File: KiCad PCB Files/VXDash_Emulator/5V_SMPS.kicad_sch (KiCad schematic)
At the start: 13 parts, among them IC1 AP62200

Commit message: Emulator board : BOM and fab prep
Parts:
- C3: MFT (none) -> Samsung Electro-Mechanics; MFT_PN (none) -> CL31B106KAHNNNE
- C4, C5, C7: MFT (none) -> Samsung Electro-Mechanics; MFT_PN (none) -> CL10B104KB8NNWC
- C6: MFT (none) -> Kyocera AVX; MFT_PN (none) -> 06035C220JAT2A
- C8, C9: MFT (none) -> Samsung Electro-Mechanics; MFT_PN (none) -> CL31B226KPHNNNE
- R42: MFT (none) -> Yageo; MFT_PN (none) -> RC0603FR-071KL
- R43: MFT (none) -> StackPole Electronics; MFT_PN (none) -> RMCF0603FT100K
- R44: MFT (none) -> Yageo; MFT_PN (none) -> RC0603FR-0743KL
- R45: MFT (none) -> Yageo; MFT_PN (none) -> RC0603FR-078K2L
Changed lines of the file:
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@@
 			)
 		)
-		(property "Description" ""
+		(property "Description" "CAP CER 22PF 50V X7R 0603"
 			(at 157.48 86.36 0)
 			(effects
@@
 			)
 		)
-		(property "MFT" ""
+		(property "MFT" "Kyocera AVX"
 			(at 157.48 86.36 0)
 			(effects
@@
 			)
 		)
-		(property "MFT_PN" ""
+		(property "MFT_PN" "06035C220JAT2A"
 			(at 157.48 86.36 0)
 			(effects
@@
 			)
 		)
-		(property "Description" ""
+		(property "Description" "CAP CER 0.1UF 50V X7R 0603"
 			(at 90.17 82.55 0)
 			(effects
@@
 			)
 		)
-		(property "MFT" ""
+		(property "MFT" "Samsung Electro-Mechanics"
 			(at 90.17 82.55 0)
 			(effects
@@
 			)
 		)
-		(property "MFT_PN" ""
+		(property "MFT_PN" "CL10B104KB8NNWC"
 			(at 90.17 82.55 0)
 			(effects
@@
 			)
 		)
-		(property "Description" ""
+		(property "Description" "CAP CER 22UF 10V X7R 1206"
 			(at 189.23 86.36 0)
 			(effects
@@
 			)
 		)
-		(property "MFT" ""
+		(property "MFT" "Samsung Electro-Mechanics"
 			(at 189.23 86.36 0)
 			(effects
@@
 			)
 		)
-		(property "MFT_PN" ""
+		(property "MFT_PN" "CL31B226KPHNNNE"
 			(at 189.23 86.36 0)
 			(effects
@@
 			)
 		)
-		(property "Description" ""
+		(property "Description" "CAP CER 22UF 10V X7R 1206"
 			(at 181.61 86.36 0)
 			(effects
@@
 			)
 		)
-		(property "MFT" ""
+		(property "MFT" "Samsung Electro-Mechanics"
 			(at 181.61 86.36 0)
 			(effects
@@
 			)
 		)
-		(property "MFT_PN" ""
+		(property "MFT_PN" "CL31B226KPHNNNE"
 			(at 181.61 86.36 0)
 			(effects
@@
 			)
 		)
-		(property "Description" ""
+		(property "Description" "RES 1K OHM 1% 1/10W 0603"
 			(at 74.93 91.44 0)
 			(effects
@@
 			)
 		)
-		(property "MFT" ""
+		(property "MFT" "Yageo"
 			(at 74.93 91.44 0)
 			(effects
@@
 			)
 		)
-		(property "MFT_PN" ""
+		(property "MFT_PN" "RC0603FR-071KL"
 			(at 74.93 91.44 0)
 			(effects
@@
 			)
 		)
-		(property "Description" ""
+		(property "Description" "FIXED IND 4.7UH 3.2A 32 MOHM SMD"
 			(at 142.24 83.82 0)
 			(effects
@@
 			)
 		)
-		(property "Description" ""
+		(property "Description" "CAP CER 0.1UF 50V X7R 0603"
 			(at 129.54 76.2 0)
 			(effects
@@
 			)
 		)
-		(property "MFT" ""
+		(property "MFT" "Samsung Electro-Mechanics"
 			(at 129.54 76.2 0)
 			(effects
@@
 			)
 		)
-		(property "MFT_PN" ""
+		(property "MFT_PN" "CL10B104KB8NNWC"
 			(at 129.54 76.2 0)
 			(effects
@@
 			)
 		)
-		(property "Description" ""
+		(property "Description" "CAP CER 0.1UF 50V X7R 0603"
 			(at 173.99 86.36 0)
 			(effects
@@
 			)
 		)
-		(property "MFT" ""
+		(property "MFT" "Samsung Electro-Mechanics"
 			(at 173.99 86.36 0)
 			(effects
@@
 			)
 		)
-		(property "MFT_PN" ""
+		(property "MFT_PN" "CL10B104KB8NNWC"
 			(at 173.99 86.36 0)
 			(effects
@@
 			)
 		)
-		(property "Description" ""
+		(property "Description" "RES 8.2K OHM 1% 1/10W 0603"
 			(at 148.59 97.79 0)
 			(effects
@@
 			)
 		)
-		(property "MFT" ""
+		(property "MFT" "Yageo"
 			(at 148.59 97.79 0)
 			(effects
@@
 			)
 		)
-		(property "MFT_PN" ""
+		(property "MFT_PN" "RC0603FR-078K2L"
 			(at 148.59 97.79 0)
 			(effects
@@
 			)
 		)
-		(property "Description" ""
+		(property "Description" "CAP CER 10UF 25V X7R 1206"
 			(at 82.55 82.55 0)
 			(effects
@@
 			)
 		)
-		(property "MFT" ""
+		(property "MFT" "Samsung Electro-Mechanics"
 			(at 82.55 82.55 0)
 			(effects
@@
 			)
 		)
-		(property "MFT_PN" ""
+		(property "MFT_PN" "CL31B106KAHNNNE"
 			(at 82.55 82.55 0)
 			(effects
@@
 			)
 		)
-		(property "Description" ""
+		(property "Description" "RES 100K OHM 1% 1/10W 0603"
 			(at 100.33 96.52 0)
 			(effects
@@
 			)
 		)
-		(property "MFT" ""
+		(property "MFT" "StackPole Electronics"
 			(at 100.33 96.52 0)
 			(effects
@@
 			)
 		)
-		(property "MFT_PN" ""
+		(property "MFT_PN" "RMCF0603FT100K"
 			(at 100.33 96.52 0)
 			(effects
@@
 			)
 		)
-		(property "Description" ""
+		(property "Description" "RES 43K OHM 1% 1/10W 0603"
 			(at 148.59 86.36 0)
 			(effects
@@
 			)
 		)
-		(property "MFT" ""
+		(property "MFT" "Yageo"
 			(at 148.59 86.36 0)
 			(effects
@@
 			)
 		)
-		(property "MFT_PN" ""
+		(property "MFT_PN" "RC0603FR-0743KL"
 			(at 148.59 86.36 0)
 			(effects

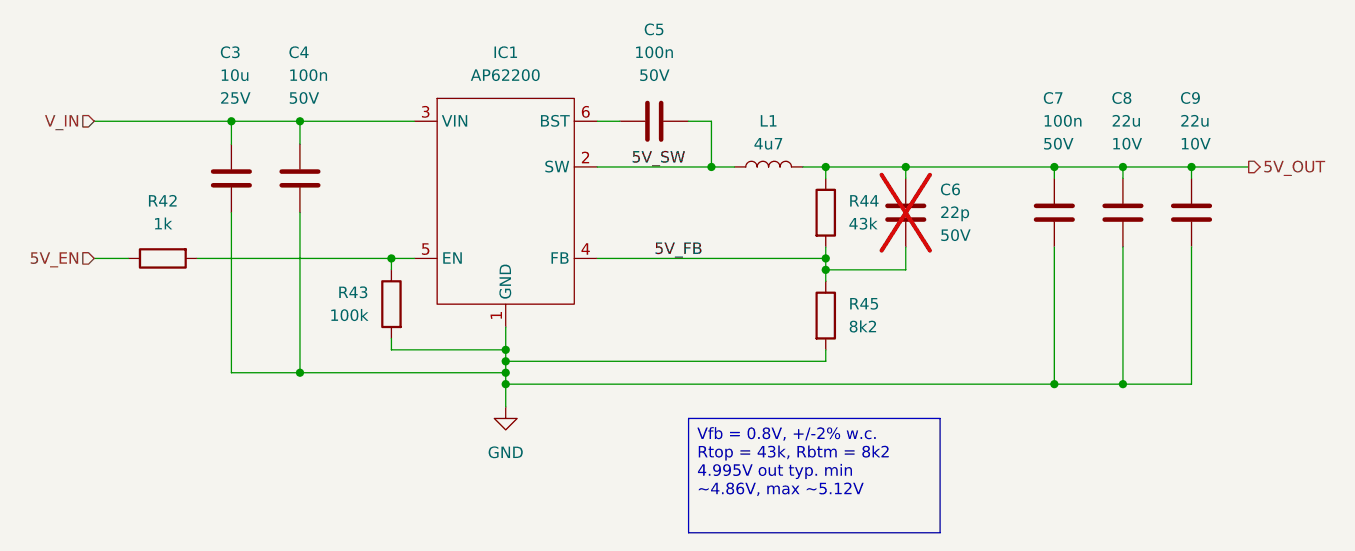
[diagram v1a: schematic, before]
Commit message: Emulator : LCSC part numbers and production files
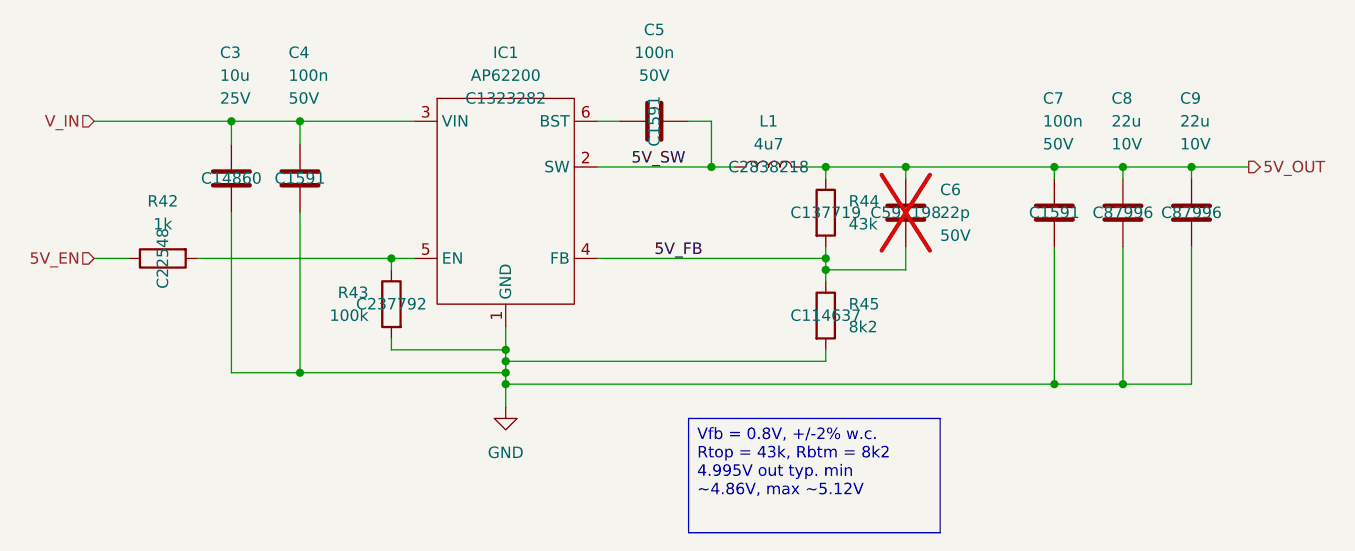
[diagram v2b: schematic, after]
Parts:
- C3: LCSC (none) -> C14860
- C4, C5, C7: LCSC (none) -> C1591; MFT_PN CL10B104KB8NNWC -> CL10B104KB8NNNC
- C6: LCSC (none) -> C597198
- C8, C9: LCSC (none) -> C87996
- IC1: LCSC (none) -> C1323282
- L1: LCSC (none) -> C2838218
- R42: LCSC (none) -> C22548
- R43: LCSC (none) -> C237792
- R44: LCSC (none) -> C137719
- R45: LCSC (none) -> C114637
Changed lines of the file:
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@@
+			)
+		)
+		(property "LCSC" "C597198"
+			(at 157.48 86.36 0)
+			(effects
+				(font
+					(size 1.27 1.27)
+				)
 			)
 		)
@@
 			)
 		)
-		(property "MFT_PN" "CL10B104KB8NNWC"
+		(property "MFT_PN" "CL10B104KB8NNNC"
 			(at 90.17 82.55 0)
 			(effects
@@
 				)
 				(hide yes)
+			)
+		)
+		(property "LCSC" "C1591"
+			(at 90.17 82.55 0)
+			(effects
+				(font
+					(size 1.27 1.27)
+				)
 			)
 		)
@@
 			)
 		)
+		(property "LCSC" "C87996"
+			(at 189.23 86.36 0)
+			(effects
+				(font
+					(size 1.27 1.27)
+				)
+			)
+		)
 		(pin "2"
 		)
@@
 				)
 				(hide yes)
+			)
+		)
+		(property "LCSC" "C87996"
+			(at 181.61 86.36 0)
+			(effects
+				(font
+					(size 1.27 1.27)
+				)
 			)
 		)
@@
 				)
 				(hide yes)
+			)
+		)
+		(property "LCSC" "C1323282"
+			(at 113.03 73.66 0)
+			(effects
+				(font
+					(size 1.27 1.27)
+				)
 			)
 		)
@@
 			)
 		)
+		(property "LCSC" "C22548"
+			(at 74.93 91.44 0)
+			(effects
+				(font
+					(size 1.27 1.27)
+				)
+			)
+		)
 		(pin "1"
 		)
@@
 				)
 				(hide yes)
+			)
+		)
+		(property "LCSC" "C2838218"
+			(at 142.24 81.28 0)
+			(effects
+				(font
+					(size 1.27 1.27)
+				)
 			)
 		)
@@
 			)
 		)
-		(property "MFT_PN" "CL10B104KB8NNWC"
+		(property "MFT_PN" "CL10B104KB8NNNC"
 			(at 129.54 76.2 0)
 			(effects
@@
 				)
 				(hide yes)
+			)
+		)
+		(property "LCSC" "C1591"
+			(at 129.54 76.2 0)
+			(effects
+				(font
+					(size 1.27 1.27)
+				)
 			)
 		)
@@
 			)
 		)
-		(property "MFT_PN" "CL10B104KB8NNWC"
+		(property "MFT_PN" "CL10B104KB8NNNC"
 			(at 173.99 86.36 0)
 			(effects
@@
 				)
 				(hide yes)
+			)
+		)
+		(property "LCSC" "C1591"
+			(at 173.99 86.36 0)
+			(effects
+				(font
+					(size 1.27 1.27)
+				)
 			)
 		)
@@
 			)
 		)
+		(property "LCSC" "C114637"
+			(at 148.59 97.79 0)
+			(effects
+				(font
+					(size 1.27 1.27)
+				)
+			)
+		)
 		(pin "1"
 		)
@@
 				)
 				(hide yes)
+			)
+		)
+		(property "LCSC" "C14860"
+			(at 82.55 82.55 0)
+			(effects
+				(font
+					(size 1.27 1.27)
+				)
 			)
 		)
@@
 			)
 		)
+		(property "LCSC" "C237792"
+			(at 100.33 96.52 0)
+			(effects
+				(font
+					(size 1.27 1.27)
+				)
+			)
+		)
 		(pin "1"
 		)
@@
 			)
 		)
+		(property "LCSC" "C137719"
+			(at 148.59 86.36 0)
+			(effects
+				(font
+					(size 1.27 1.27)
+				)
+			)
+		)

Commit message: Emulator : Updating BOM with LCSC alts
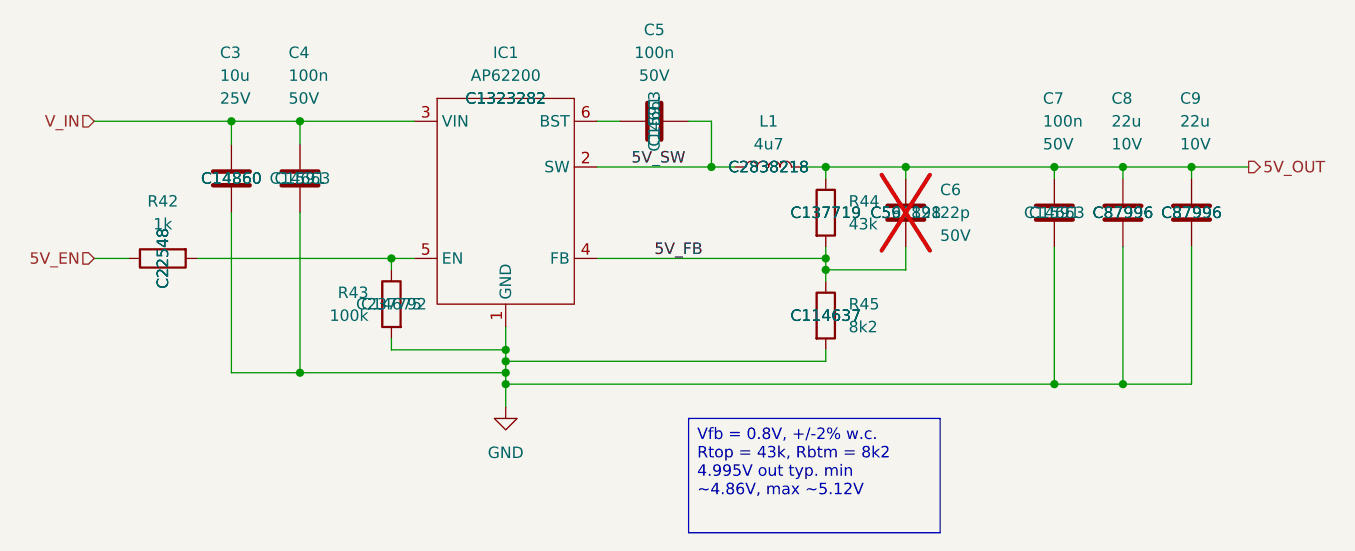
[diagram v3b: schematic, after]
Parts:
- C3: LCSC alt (none) -> C14860
- C4, C5, C7: LCSC alt (none) -> C14663
- C6: LCSC alt (none) -> C561821
- C8, C9: LCSC alt (none) -> C87996
- IC1: LCSC alt (none) -> C1323282
- L1: LCSC alt (none) -> C2838218
- R42: LCSC alt (none) -> C22548
- R43: LCSC alt (none) -> C14675
- R44: LCSC alt (none) -> C137719
- R45: LCSC alt (none) -> C114637
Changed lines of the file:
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@@
+			)
+		)
+		(property "LCSC alt" "C561821"
+			(at 157.48 86.36 0)
+			(effects
+				(font
+					(size 1.27 1.27)
+				)
 			)
 		)
@@
 			)
 		)
+		(property "LCSC alt" "C14663"
+			(at 90.17 82.55 0)
+			(effects
+				(font
+					(size 1.27 1.27)
+				)
+			)
+		)
 		(pin "1"
 		)
@@
 			)
 		)
+		(property "LCSC alt" "C87996"
+			(at 189.23 86.36 0)
+			(effects
+				(font
+					(size 1.27 1.27)
+				)
+			)
+		)
 		(pin "2"
 		)
@@
 		)
 		(property "LCSC" "C87996"
+			(at 181.61 86.36 0)
+			(effects
+				(font
+					(size 1.27 1.27)
+				)
+			)
+		)
+		(property "LCSC alt" "C87996"
 			(at 181.61 86.36 0)
 			(effects
@@
 		)
 		(property "LCSC" "C1323282"
+			(at 113.03 73.66 0)
+			(effects
+				(font
+					(size 1.27 1.27)
+				)
+			)
+		)
+		(property "LCSC alt" "C1323282"
 			(at 113.03 73.66 0)
 			(effects
@@
 			)
 		)
+		(property "LCSC alt" "C22548"
+			(at 74.93 91.44 0)
+			(effects
+				(font
+					(size 1.27 1.27)
+				)
+			)
+		)
 		(pin "1"
 		)
@@
 		)
 		(property "LCSC" "C2838218"
+			(at 142.24 81.28 0)
+			(effects
+				(font
+					(size 1.27 1.27)
+				)
+			)
+		)
+		(property "LCSC alt" "C2838218"
 			(at 142.24 81.28 0)
 			(effects
@@
 			)
 		)
+		(property "LCSC alt" "C14663"
+			(at 129.54 76.2 0)
+			(effects
+				(font
+					(size 1.27 1.27)
+				)
+			)
+		)
 		(pin "1"
 		)
@@
 			)
 		)
+		(property "LCSC alt" "C14663"
+			(at 173.99 86.36 0)
+			(effects
+				(font
+					(size 1.27 1.27)
+				)
+			)
+		)
 		(pin "1"
 		)
@@
 			)
 		)
+		(property "LCSC alt" "C114637"
+			(at 148.59 97.79 0)
+			(effects
+				(font
+					(size 1.27 1.27)
+				)
+			)
+		)
 		(pin "1"
 		)
@@
 		)
 		(property "LCSC" "C14860"
+			(at 82.55 82.55 0)
+			(effects
+				(font
+					(size 1.27 1.27)
+				)
+			)
+		)
+		(property "LCSC alt" "C14860"
 			(at 82.55 82.55 0)
 			(effects
@@
 			)
 		)
+		(property "LCSC alt" "C14675"
+			(at 100.33 96.52 0)
+			(effects
+				(font
+					(size 1.27 1.27)
+				)
+			)
+		)
 		(pin "1"
 		)
@@
 			(at 148.59 86.36 0)
 			(effects
+				(font
+					(size 1.27 1.27)
+				)
+			)
+		)
+		(property "LCSC alt" "C137719"
+			(at 148.59 86.36 0)
+			(effects
